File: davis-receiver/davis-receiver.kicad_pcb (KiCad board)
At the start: 4 copper layers, 146 parts, among them J1 Conn_Coaxial, J2 Wurth_74982104400, J3 JTAG, J4 UART, J5 SPI-BARO, J6 SPI-RF, Q1 FDC2512, SW1 MCU_RESET, T1 POE70P-33, U1 TM4C129ENCZADI3R, U2 CC1125RHBR, U3 FXPS7115D4, U4 TPS79930DDCR, U5 MB10S, U6 MB10S, U7 TPS23753A, U8 FOD817A3SD, U9 TLV431ACDBZR, X1 ECS-2520MV-400-AY-TR, Y1 LFXTAL071758CUTT

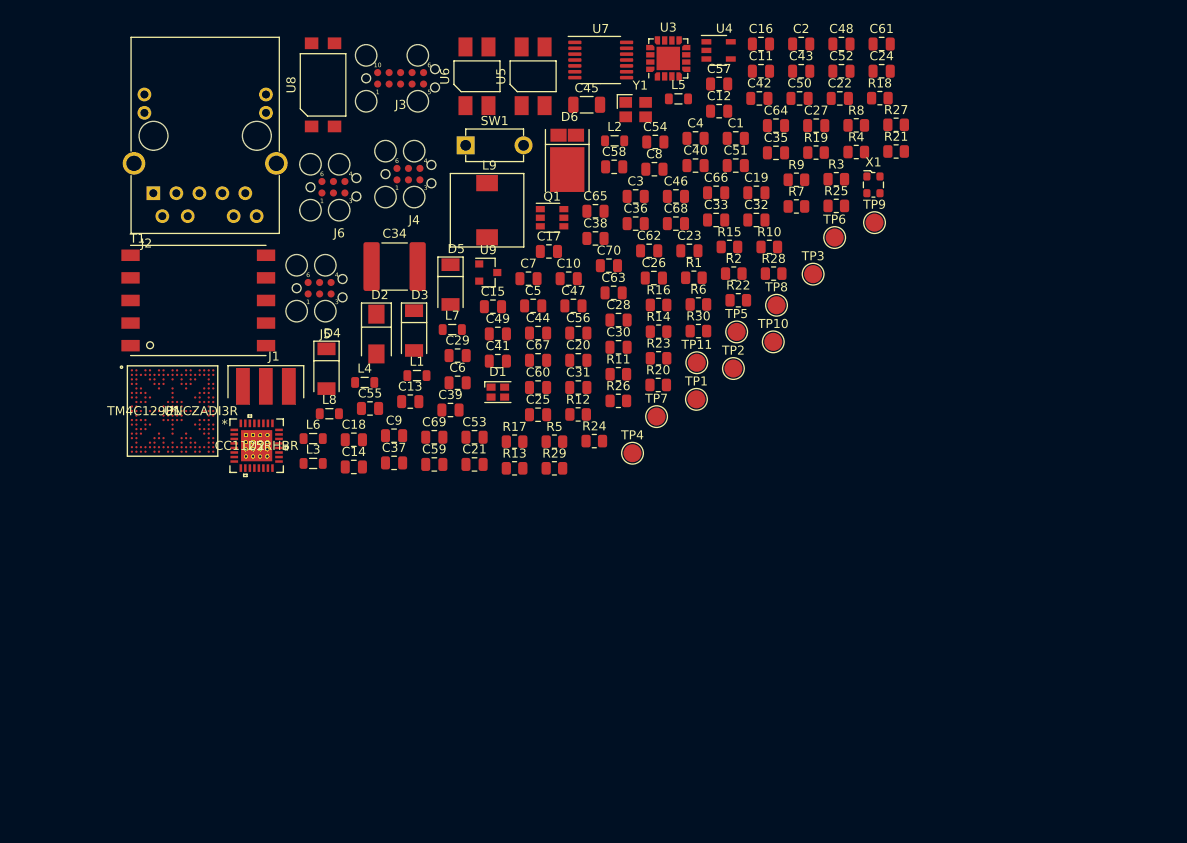
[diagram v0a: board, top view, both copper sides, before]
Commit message: Davis Receiver v1.0
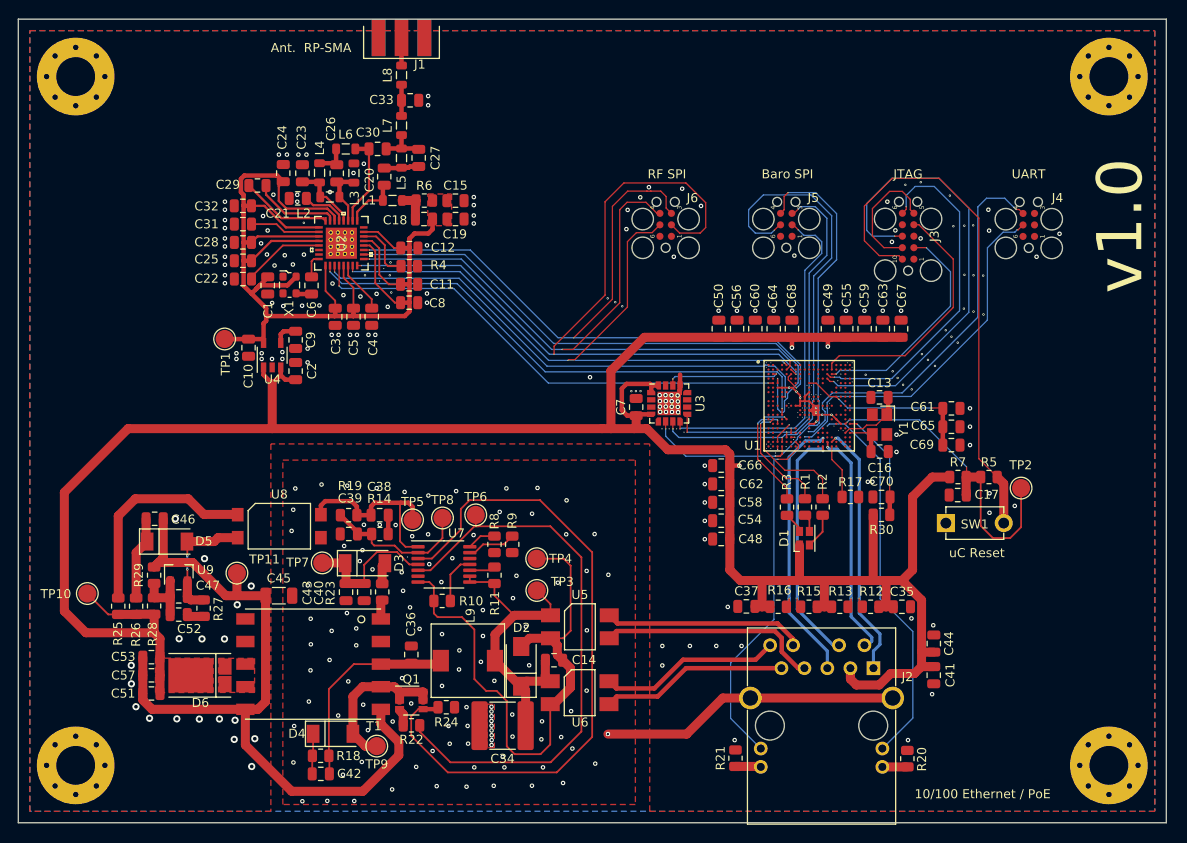
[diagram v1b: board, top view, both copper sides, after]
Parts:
- added H1: MountingHole, MountingHole:MountingHole_4.3mm_M4_Pad_Via, F.Cu at (145.3, 107.2)
- added H2: MountingHole, MountingHole:MountingHole_4.3mm_M4_Pad_Via, F.Cu at (31.1, 31.1)
- added H3: MountingHole, MountingHole:MountingHole_4.3mm_M4_Pad_Via, F.Cu at (31.1, 107.2)
- added H4: MountingHole, MountingHole:MountingHole_4.3mm_M4_Pad_Via, F.Cu at (145.3, 31.1)
- C1, C2, C35, C37, C41, C44, C7: value 100nF -> 0.1uF
- C11, C12, C22, C25, C28, C3, C31, C32, C5, C8: value 47nF -> 0.047uF
- C15, C9: value 10nF -> 0.01uF
- C52: value 6.8nF -> 6800pF
- U2: value CC1125RHBR -> RHB32_3P45X3P45_TEX
- moved R18 95.5 mm to (58.1, 106.2), turned to 180 degrees
- moved C52 94.8 mm to (42.4, 90.6), turned to 180 degrees
- moved J2 94.4 mm to (113.6, 102.9), turned to 180 degrees
- moved R27 93.4 mm to (45.2, 89.9), turned to 90 degrees
- moved R25 90.9 mm to (35.8, 89.6), turned to 270 degrees
- moved C57 90.7 mm to (39.4, 97.3), turned to 180 degrees
- moved C42 89.1 mm to (58.2, 108.2), turned to 180 degrees
- moved C51 87.1 mm to (39.4, 99.3), turned to 180 degrees
- moved TP10 80.8 mm to (32.3, 88.2), turned to 180 degrees
- moved TP9 79.9 mm to (64.4, 105.1), turned to 180 degrees
- moved R28 77.8 mm to (39.7, 89.6), turned to 270 degrees
- moved C43 76.5 mm to (61.0, 88.1), turned to 270 degrees
- moved U1 70.4 mm to (112.2, 67.5)
- moved D6 70.4 mm to (46.6, 97.3), turned to 270 degrees
- moved R21 69.4 mm to (104.0, 106.5), turned to 90 degrees
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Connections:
- net Net-(J2-Pad1) renamed /ETH_TX_P
- net Net-(J2-Pad2) renamed /ETH_TX_N
- net Net-(J2-Pad4) renamed /ETH_RX_P
- net Net-(J2-Pad5) renamed /ETH_RX_N
- J2 pad SHD: GND -> GND1
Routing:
- net +3V3: track 0.00 -> 327.3 mm, vias 0 -> 11
- net +3V0: track 0.00 -> 138.5 mm
- net /RF_SCLK: track 0.00 -> 93.7 mm, vias 0 -> 3
- net GND: track 0.00 -> 86.2 mm, vias 0 -> 225
- net /RF_CS: track 0.00 -> 83.7 mm, vias 0 -> 3
- net /RF_MISO: track 0.00 -> 77.0 mm, vias 0 -> 3
- net Net-(Q1-Pad4): track 0.00 -> 75.0 mm
- net /RF_MOSI: track 0.00 -> 73.6 mm, vias 0 -> 3
- net Net-(R22-Pad1): track 0.00 -> 63.7 mm
- net /RF_GPIO0: track 0.00 -> 63.7 mm, vias 0 -> 2
- net Net-(C14-Pad2): track 0.00 -> 62.1 mm
- net /RF_RESET: track 0.00 -> 59.7 mm, vias 0 -> 2
- net /JTAG_RESET: track 0.00 -> 59.5 mm
- net /BAR_MOSI: track 0.00 -> 58.4 mm, vias 0 -> 3
- net /RF_GPIO3: track 0.00 -> 58.1 mm, vias 0 -> 2
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- added copper zone on F.Cu, net +3V0
- added copper zone on F.Cu, net +3V3
- added copper zone on B.Cu, net GND
- added copper zone on F.Cu, net GND
- added copper zone on In1.Cu, net GND
- added copper zone on In2.Cu, net GND
- added copper zone on F.Cu, net GND1
- added copper zone on In1.Cu, net GND1
- added copper zone on F.Cu, net Net-(D6-Pad2)
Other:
- board outline added: 127 x 88.9 mm
- net class Default: clearance 0.2 -> 0.127
- net class ENET added: clearance 0.127, trace_width 0.25, via_dia 0.8, via_drill 0.4
- rule trace_clearance: 0.2 -> 0.127
- rule trace_min: 0.2 -> 0.127
- rule via_min_drill: 0.3 -> 0.0508
- rule via_min_size: 0.4 -> 0.1016
- board text added: "10/100 Ethernet / PoE"
- board text added: "Ant. RP-SMA"
- board text added: "Baro SPI"
- board text added: "Davis Receiver"
- board text added: "JTAG"
- board text added: "RF SPI"
- board text added: "UART"
- board text added: "uC Reset"
- board text added: "v1.0"
